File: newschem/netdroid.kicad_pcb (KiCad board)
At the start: 2 copper layers, 49 x 74 mm, 62 parts, among them P1 CONN_1, P2 CONN_1, P3 CONN_1, P4 CONN_1, P5 CONN_1, P6 CONN_1, P7 CONN_1, P8 CONN_1, U1 STM32F100C4

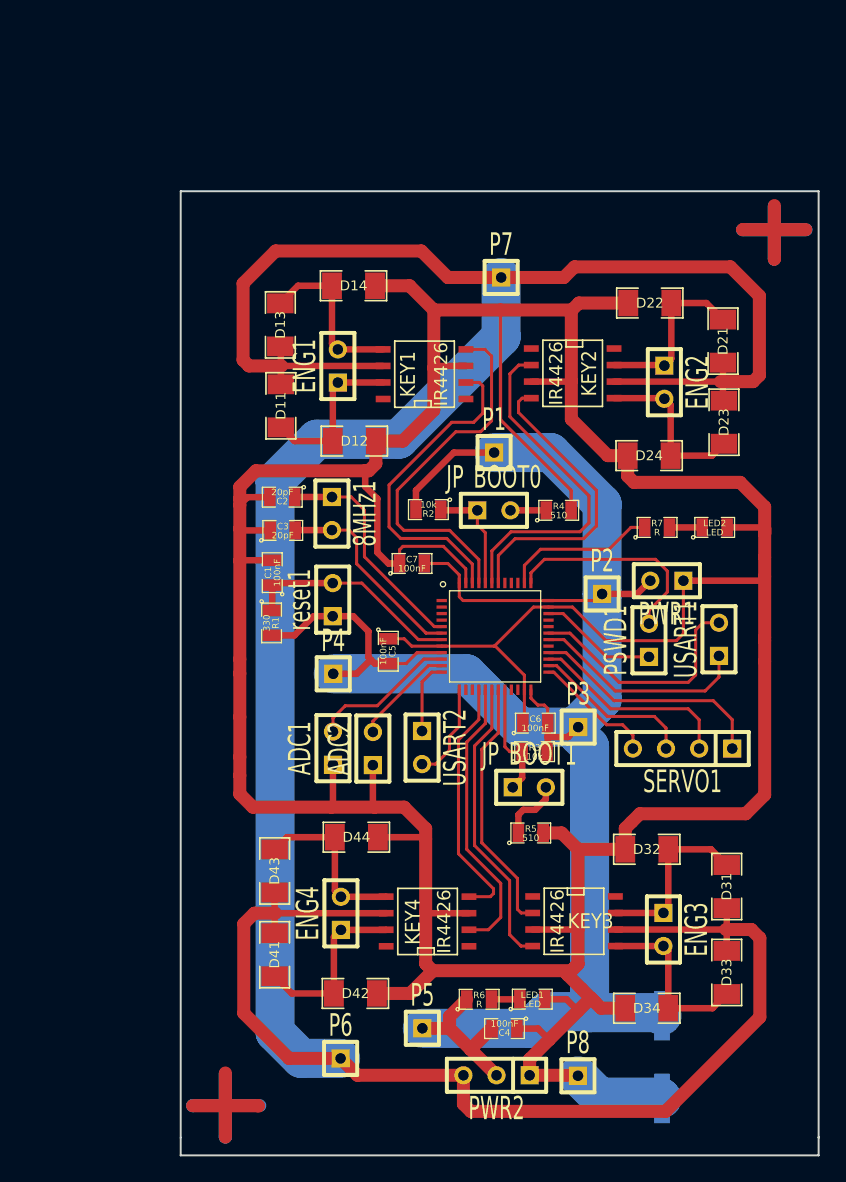
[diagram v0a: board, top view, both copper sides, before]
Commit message: Надеюсь, это финальная версия
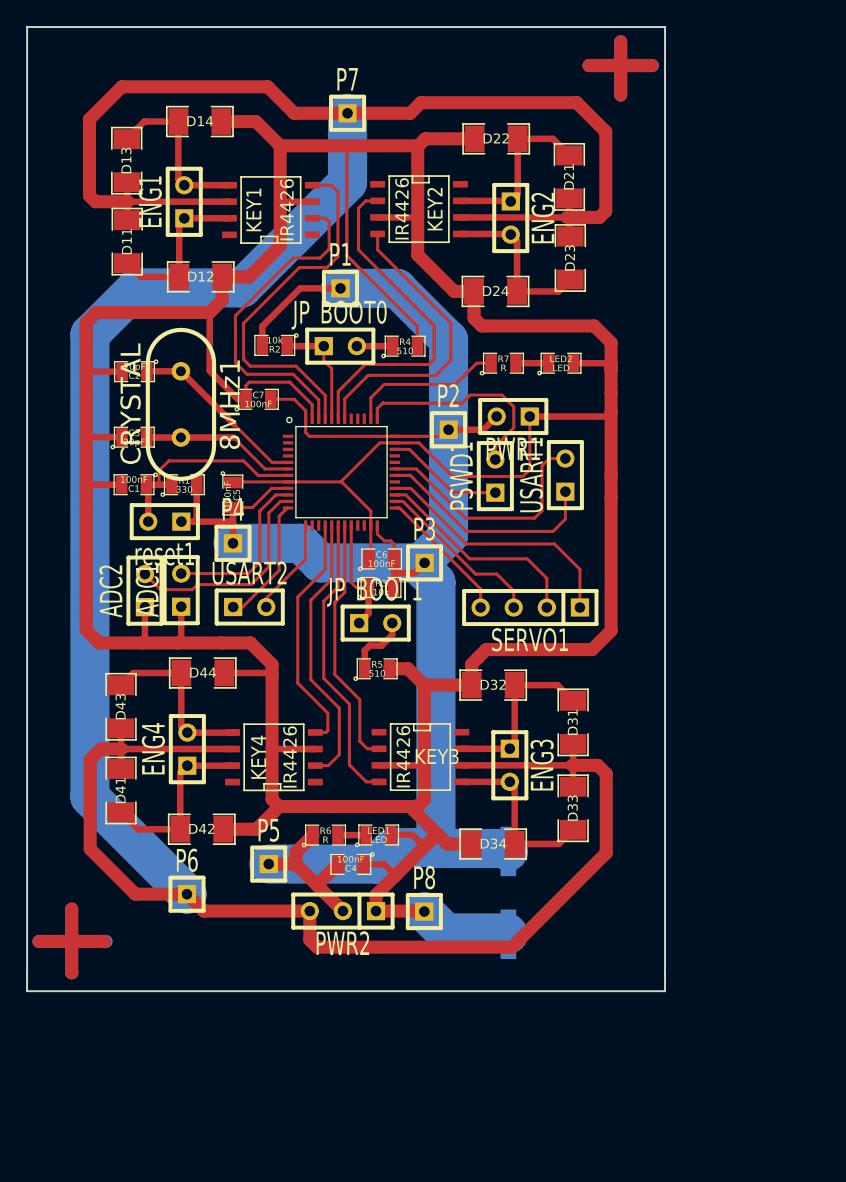
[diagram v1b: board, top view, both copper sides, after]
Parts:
- 8MHz1: footprint SIL-2 -> HC-49V
- moved ADC2 21.3 mm to (27.4, 62.2)
- moved D24 17.3 mm to (54.3, 39.2)
- moved D43 17.3 mm to (25.5, 71.1)
- moved ENG3 17.3 mm to (55.4, 75.6)
- moved R7 17.3 mm to (54.9, 44.7)
- moved KEY3 17.3 mm to (48.5, 74.9)
- moved R2 17.3 mm to (37.3, 43.4)
- moved R5 17.3 mm to (45.2, 68.2)
- moved U1 17.3 mm to (42.4, 53.1)
- moved C9 17.3 mm to (55.2, 85.4)
- moved C7 17.3 mm to (36.1, 47.5)
- moved D11 17.3 mm to (26.0, 35.4)
- moved D12 17.3 mm to (31.6, 38.1)
- moved D13 17.3 mm to (26.0, 29.2)
- moved D14 17.3 mm to (31.6, 26.2)
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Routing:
- net VDD: track 159.4 -> 148.5 mm
- net N-0000021: track 7.87 -> 16.7 mm
- net N-0000017: track 5.58 -> 9.80 mm
- net N-0000039: track 15.7 -> 11.9 mm
- net N-0000061: track 17.5 -> 19.5 mm
- net N-0000020: track 11.3 -> 13.0 mm
- net +12V: track 247.1 -> 248.3 mm
- net N-0000011: track 18.4 -> 19.7 mm
- net N-0000012: track 9.51 -> 10.6 mm
- net N-0000014: track 15.7 -> 16.5 mm
- net N-000008: track 19.4 -> 18.6 mm
- net N-000001: track 23.7 -> 22.9 mm
- net N-0000013: track 12.6 -> 13.2 mm
- net N-000007: track 22.0 -> 21.3 mm
- net N-0000025: track 16.8 -> 17.4 mm
